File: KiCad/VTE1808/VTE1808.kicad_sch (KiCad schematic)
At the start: 32 parts, among them J1 Program, J2 Display, J3 Power, M1 Stepper_Motor, SW1 Switch, SW5 SW_Push, SW6 SW_Push, SW7 SW_Push, SW8 Reset, U1 AMS1117-5.0, U2 ATmega328P-P, U3 DS1307+, U5 ULN2003, Y1 16MHz, Y2 32.768kHz

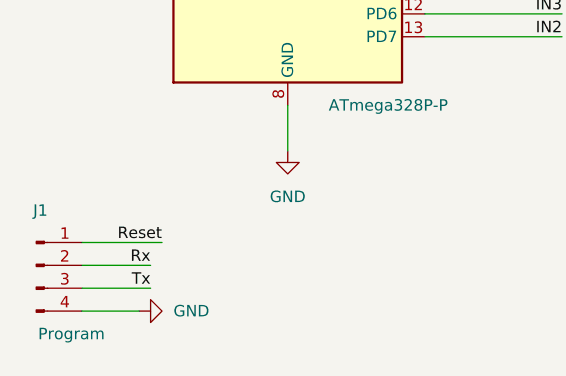
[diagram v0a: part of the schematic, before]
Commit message: latest updated
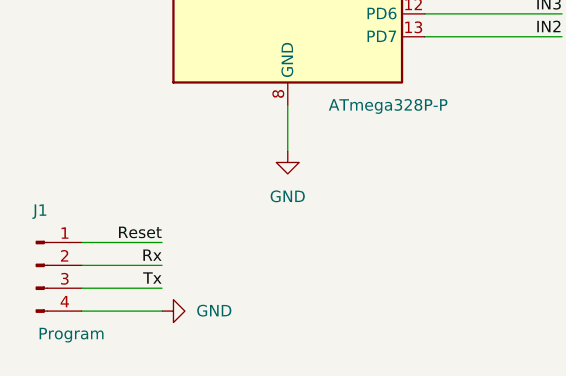
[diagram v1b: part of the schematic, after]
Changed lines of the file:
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@@
 	(wire
 		(pts
-			(xy 30.48 186.69) (xy 36.83 186.69)
+			(xy 30.48 186.69) (xy 39.37 186.69)
 		)
 		(stroke
@@
 	(wire
 		(pts
-			(xy 30.48 184.15) (xy 38.1 184.15)
+			(xy 30.48 184.15) (xy 39.37 184.15)
 		)
 		(stroke
@@
 	(wire
 		(pts
-			(xy 30.48 181.61) (xy 38.1 181.61)
+			(xy 30.48 181.61) (xy 39.37 181.61)
 		)
 		(stroke
@@
 	)
 	(label "Tx"
-		(at 38.1 184.15 180)
+		(at 39.37 184.15 180)
 		(fields_autoplaced yes)
 		(effects
@@
 	)
 	(label "Rx"
-		(at 38.1 181.61 180)
+		(at 39.37 181.61 180)
 		(fields_autoplaced yes)
 		(effects
@@
 	(symbol
 		(lib_id "power:GND")
-		(at 36.83 186.69 90)
+		(at 39.37 186.69 90)
 		(unit 1)
 		(exclude_from_sim no)
@@
 		(fields_autoplaced yes)
 		(property "Reference" "#PWR03"
-			(at 43.18 186.69 0)
+			(at 45.72 186.69 0)
 			(effects
 				(font
@@
 		)
 		(property "Value" "GND"
-			(at 40.64 186.6899 90)
+			(at 43.18 186.6899 90)
 			(effects
 				(font
@@
 		)
 		(property "Footprint" ""
-			(at 36.83 186.69 0)
+			(at 39.37 186.69 0)
 			(effects
 				(font
@@
 		)
 		(property "Datasheet" ""
-			(at 36.83 186.69 0)
+			(at 39.37 186.69 0)
 			(effects
 				(font
@@
 		)
 		(property "Description" "Power symbol creates a global label with name \"GND\" , ground"
-			(at 36.83 186.69 0)
+			(at 39.37 186.69 0)
 			(effects
 				(font
